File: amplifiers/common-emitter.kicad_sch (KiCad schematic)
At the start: 10 parts, among them Q2 Q_NPN

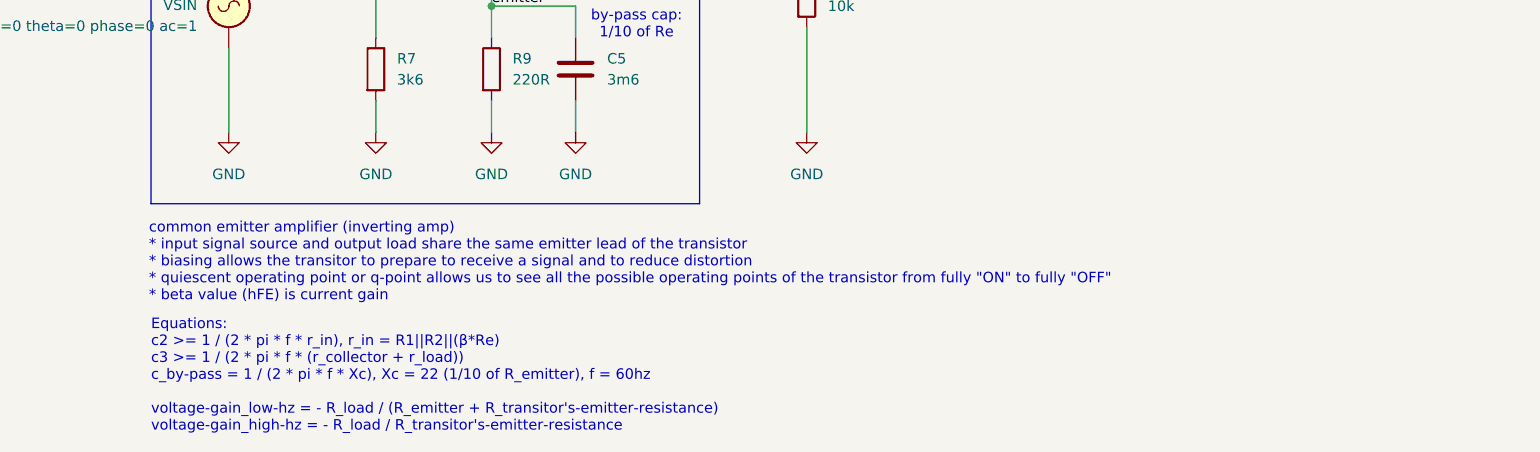
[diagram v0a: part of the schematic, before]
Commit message: wip save
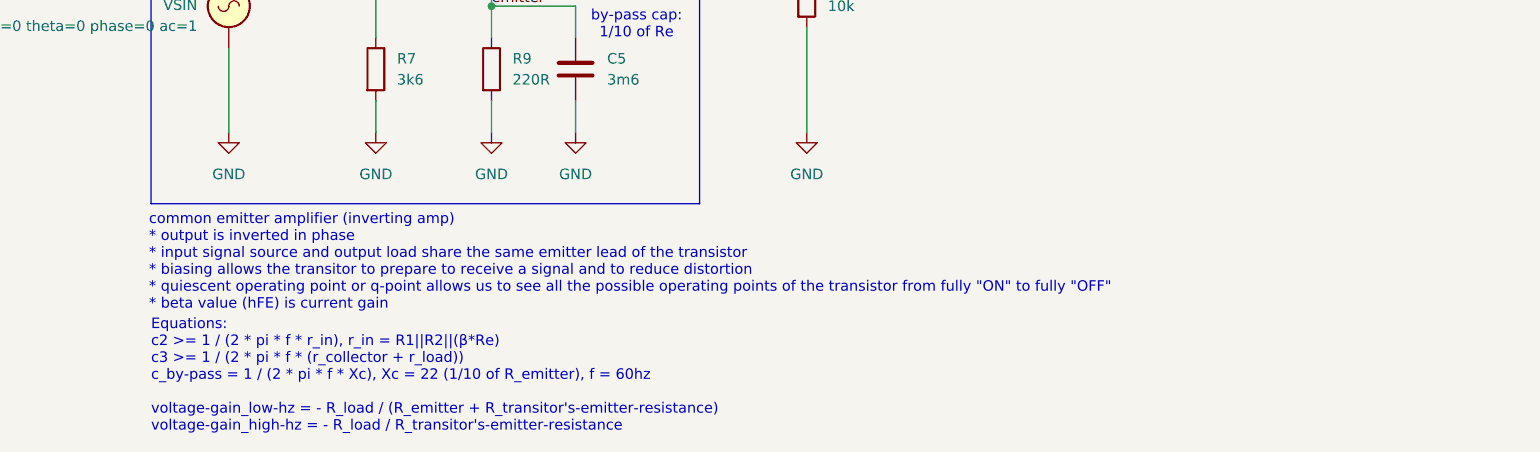
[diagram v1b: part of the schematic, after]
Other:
- note added: "common emitter amplifier (inverting amp) * output is inverted in phase * input signal source and output load share the same emitter lead of the transistor * biasing allows the transitor to prepare to receive a signal and to reduce distortion * quiescent operating point or q-point allows us to see all the possible operating points of the transistor from fully "ON" to fully "OFF" * beta value (hFE)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"
- note removed: "common emitter amplifier (inverting amp) * input signal source and output load share the same emitter lead of the transistor * biasing allows the transitor to prepare to receive a signal and to reduce distortion * quiescent operating point or q-point allows us to see all the possible operating points of the transistor from fully "ON" to fully "OFF" * beta value (hFE) is current gain"
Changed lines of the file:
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@@
 		)
 	)
-	(text "common emitter amplifier (inverting amp)\n* input signal source and output load share the same emitter lead of the transistor\n* biasing allows the transitor to prepare to receive a signal and to reduce distortion\n* quiescent operating point or q-point allows us to see all the possible operating points of the transistor from fully \"ON\" to fully \"OFF\"\n* beta value (hFE) is current gain"
+	(text "common emitter amplifier (inverting amp)\n* output is inverted in phase\n* input signal source and output load share the same emitter lead of the transistor\n* biasing allows the transitor to prepare to receive a signal and to reduce distortion\n* quiescent operating point or q-point allows us to see all the possible operating points of the transistor from fully \"ON\" to fully \"OFF\"\n* beta value (hFE) is current gain"
 		(exclude_from_sim no)
 		(at 95.758 127.508 0)
@@
 		)
 		(instances
-			(project "bjt-amp"
+			(project "amplifiers"
 				(path "/8ae523d0-1e44-401a-8c0a-127d68e06c6a/1d608d62-6b62-4129-9bf9-6774aa7c774c"
 					(reference "C4")
@@
 		)
 		(instances
-			(project "bjt-amp"
+			(project "amplifiers"
 				(path "/8ae523d0-1e44-401a-8c0a-127d68e06c6a/1d608d62-6b62-4129-9bf9-6774aa7c774c"
 					(reference "#PWR013")
@@
 		)
 		(instances
-			(project "bjt-amp"
+			(project "amplifiers"
 				(path "/8ae523d0-1e44-401a-8c0a-127d68e06c6a/1d608d62-6b62-4129-9bf9-6774aa7c774c"
 					(reference "Q2")
@@
 		)
 		(instances
-			(project "bjt-amp"
+			(project "amplifiers"
 				(path "/8ae523d0-1e44-401a-8c0a-127d68e06c6a/1d608d62-6b62-4129-9bf9-6774aa7c774c"
 					(reference "C5")
@@
 		)
 		(instances
-			(project "bjt-amp"
+			(project "amplifiers"
 				(path "/8ae523d0-1e44-401a-8c0a-127d68e06c6a/1d608d62-6b62-4129-9bf9-6774aa7c774c"
 					(reference "#PWR010")
@@
 		)
 		(instances
-			(project "bjt-amp"
+			(project "amplifiers"
 				(path "/8ae523d0-1e44-401a-8c0a-127d68e06c6a/1d608d62-6b62-4129-9bf9-6774aa7c774c"
 					(reference "R10")
@@
 		)
 		(instances
-			(project "bjt-amp"
+			(project "amplifiers"
 				(path "/8ae523d0-1e44-401a-8c0a-127d68e06c6a/1d608d62-6b62-4129-9bf9-6774aa7c774c"
 					(reference "R8")
@@
 		)
 		(instances
-			(project "bjt-amp"
+			(project "amplifiers"
 				(path "/8ae523d0-1e44-401a-8c0a-127d68e06c6a/1d608d62-6b62-4129-9bf9-6774aa7c774c"
 					(reference "R9")
@@
 		)
 		(instances
-			(project "bjt-amp"
+			(project "amplifiers"
 				(path "/8ae523d0-1e44-401a-8c0a-127d68e06c6a/1d608d62-6b62-4129-9bf9-6774aa7c774c"
 					(reference "V2")
@@
 		)
 		(instances
-			(project "bjt-amp"
+			(project "amplifiers"
 				(path "/8ae523d0-1e44-401a-8c0a-127d68e06c6a/1d608d62-6b62-4129-9bf9-6774aa7c774c"
 					(reference "C6")
@@
 		)
 		(instances
-			(project "bjt-amp"
+			(project "amplifiers"
 				(path "/8ae523d0-1e44-401a-8c0a-127d68e06c6a/1d608d62-6b62-4129-9bf9-6774aa7c774c"
 					(reference "R7")
@@
 		)
 		(instances
-			(project "bjt-amp"
+			(project "amplifiers"
 				(path "/8ae523d0-1e44-401a-8c0a-127d68e06c6a/1d608d62-6b62-4129-9bf9-6774aa7c774c"
 					(reference "#PWR08")
@@
 		)
 		(instances
-			(project "bjt-amp"
+			(project "amplifiers"
 				(path "/8ae523d0-1e44-401a-8c0a-127d68e06c6a/1d608d62-6b62-4129-9bf9-6774aa7c774c"
 					(reference "#PWR014")
@@
 		)
 		(instances
-			(project "bjt-amp"
+			(project "amplifiers"
 				(path "/8ae523d0-1e44-401a-8c0a-127d68e06c6a/1d608d62-6b62-4129-9bf9-6774aa7c774c"
 					(reference "#PWR012")
@@
 		)
 		(instances
-			(project "bjt-amp"
+			(project "amplifiers"
 				(path "/8ae523d0-1e44-401a-8c0a-127d68e06c6a/1d608d62-6b62-4129-9bf9-6774aa7c774c"
 					(reference "#PWR09")
@@
 		)
 		(instances
-			(project "bjt-amp"
+			(project "amplifiers"
 				(path "/8ae523d0-1e44-401a-8c0a-127d68e06c6a/1d608d62-6b62-4129-9bf9-6774aa7c774c"
 					(reference "#PWR011")
@@
 		)
 		(instances
-			(project "bjt-amp"
+			(project "amplifiers"
 				(path "/8ae523d0-1e44-401a-8c0a-127d68e06c6a/1d608d62-6b62-4129-9bf9-6774aa7c774c"
 					(reference "R6")
